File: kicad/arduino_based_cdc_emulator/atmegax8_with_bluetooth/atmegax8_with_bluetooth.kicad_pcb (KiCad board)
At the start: 2 copper layers, 40.9 x 35.7 mm, 66 parts, among them IC1 ATMEGA88-A, P1 CONN_9, P2 SPI, Q1 BC817-40, U1 78L05, U2 S3860M-S, U3 LM358, X1 16MHz

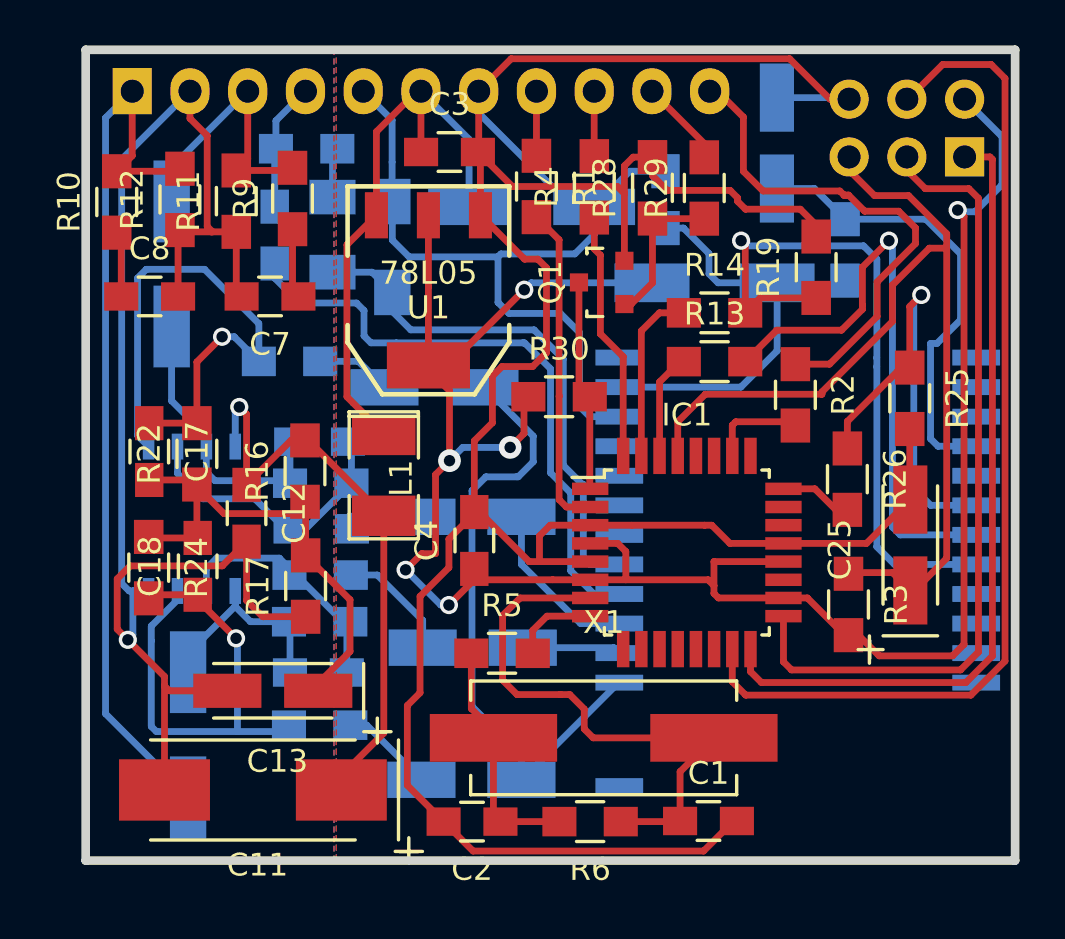
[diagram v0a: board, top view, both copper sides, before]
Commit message: updates, I do not remember what I changed ....
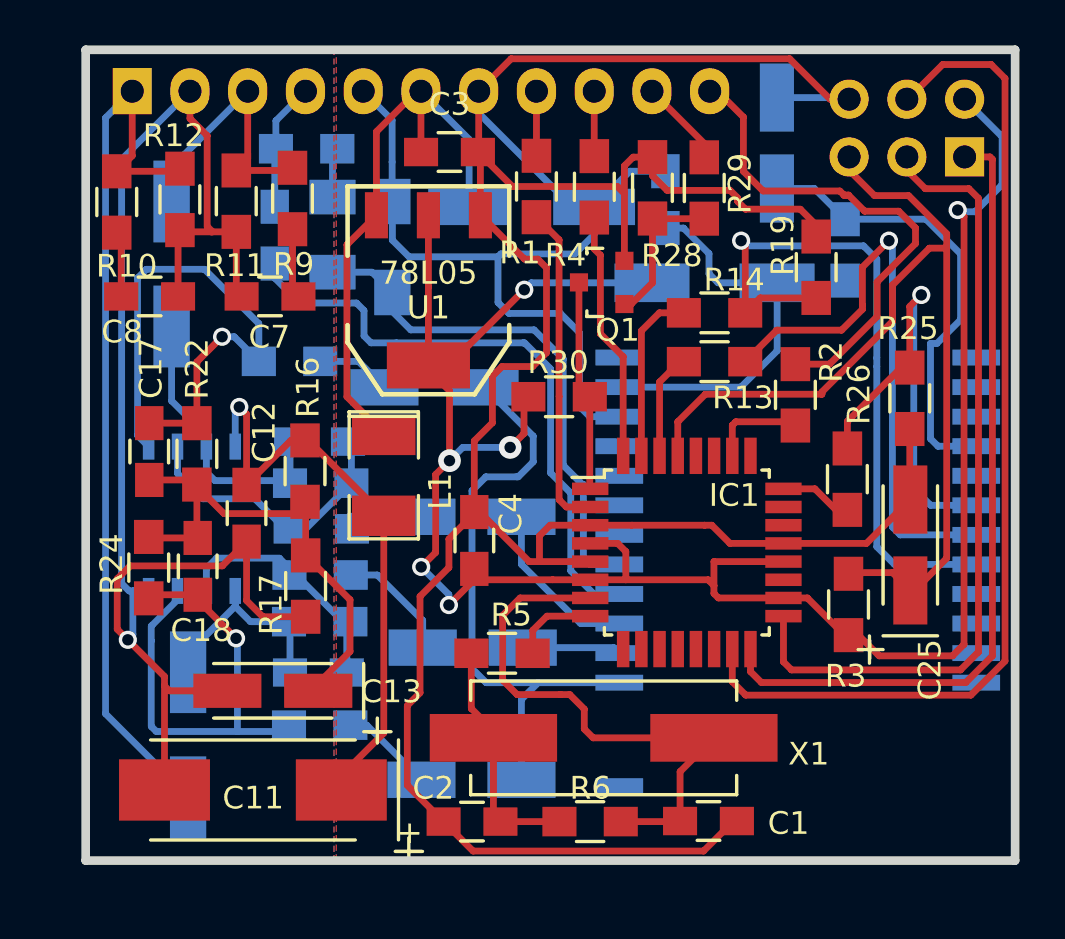
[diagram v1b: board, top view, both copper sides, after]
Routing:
- net +5V: track 95.4 -> 94.3 mm
- net /BTAGND: track 27.1 -> 26.5 mm
